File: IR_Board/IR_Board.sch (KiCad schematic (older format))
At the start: 16 parts, among them J1 Conn_02x08_Row_Letter_First, U1 TSSP58038, U10 TSSP58038, U11 TSSP58038, U12 TSSP58038, U13 TSSP58038, U14 TSSP58038, U2 TSSP58038, U3 TSSP58038, U4 TSSP58038, U5 TSSP58038, U6 TSSP58038, U7 TSSP58038, U8 TSSP58038, U9 TSSP58038

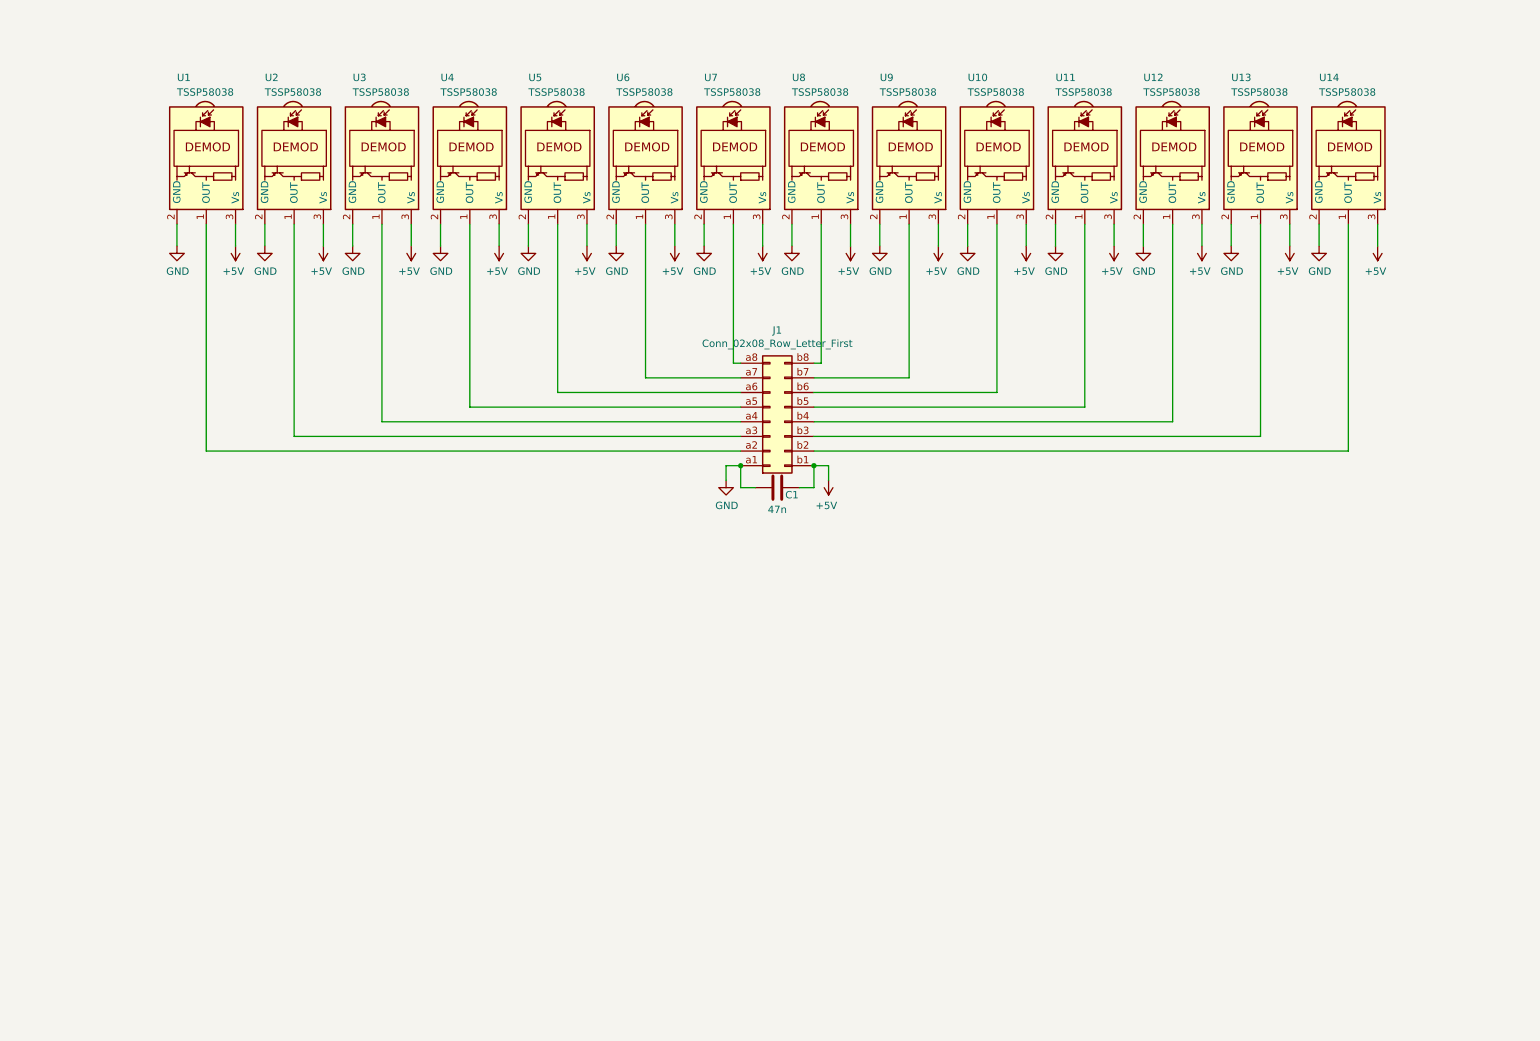
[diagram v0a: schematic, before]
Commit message: Started Light PCB
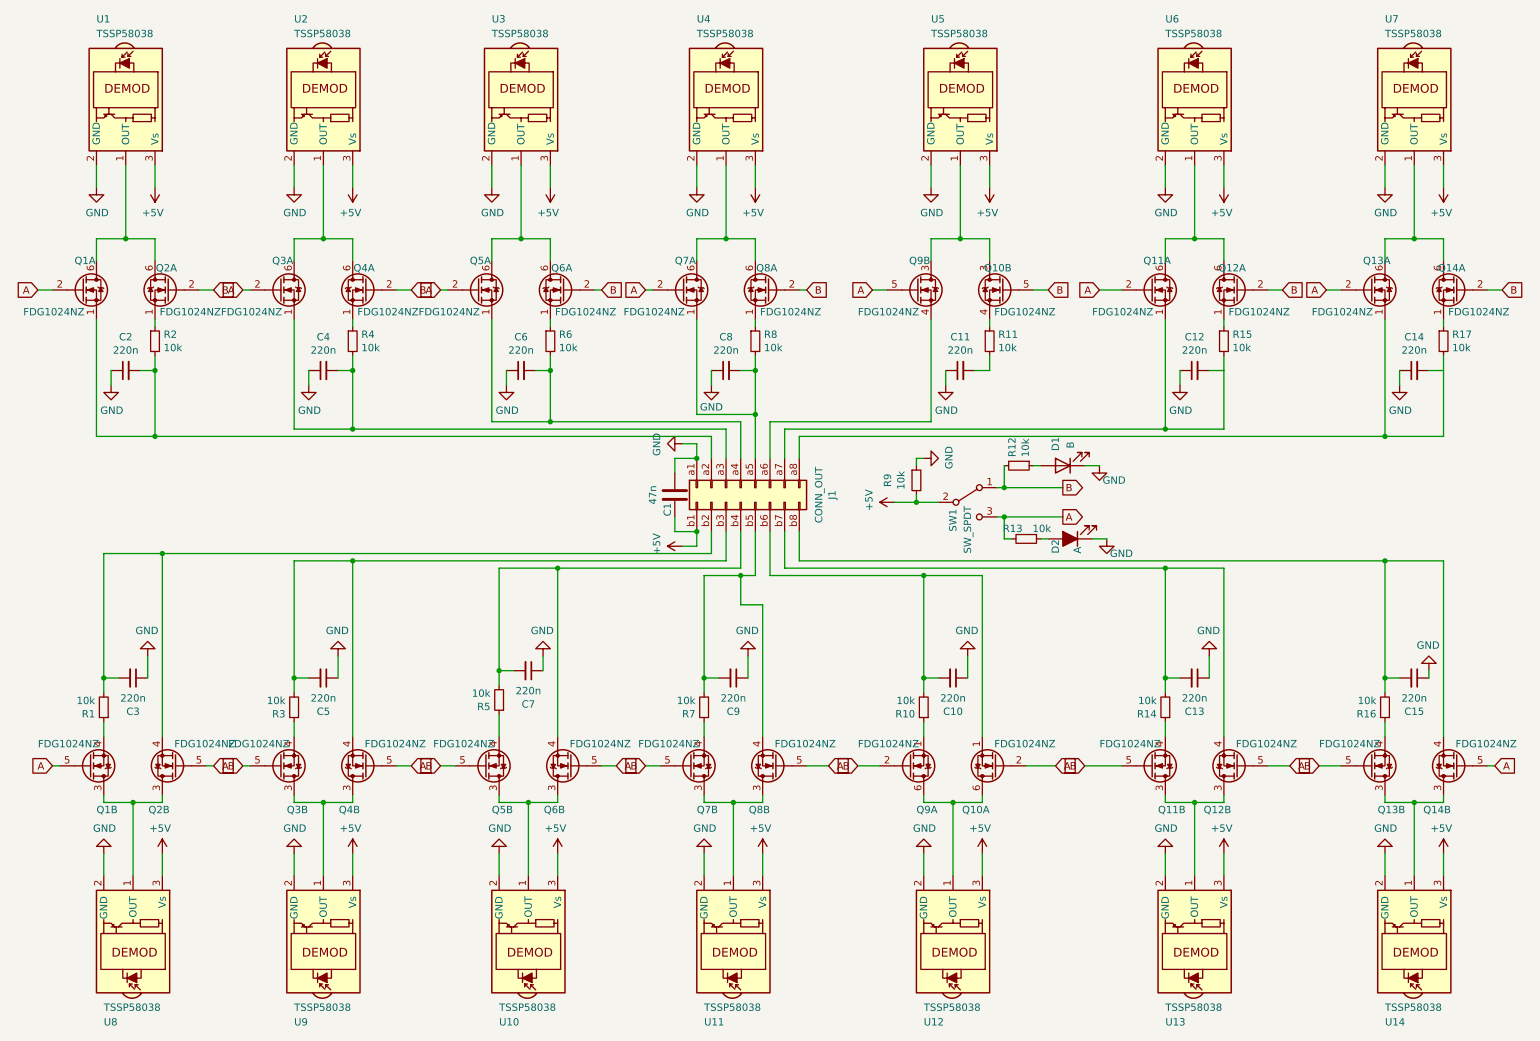
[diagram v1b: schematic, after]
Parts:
- added C10, C11, C12, C13, C14, C15, C2, C3, C4, C5, C6, C7, C8, C9: 220n, Capacitor_SMD:C_0603_1608Metric_Pad1.08x0.95mm_HandSolder, symbol Device:C_Small
- added D1: B, LED_SMD:LED_0805_2012Metric_Pad1.15x1.40mm_HandSolder, symbol Device:LED
- added D2: A, LED_SMD:LED_0805_2012Metric_Pad1.15x1.40mm_HandSolder, symbol Device:LED_ALT
- added Q1, Q10, Q11, Q12, Q13, Q14, Q2, Q3, Q4, Q5, Q6, Q7, Q8, Q9: FDG1024NZ, Package_TO_SOT_SMD:SOT-363_SC-70-6, symbol Transistor_FET:FDG1024NZ
- added R1, R10, R11, R12, R13, R14, R15, R16, R17, R2, R3, R4, R5, R6, R7, R8, R9: 10k, Resistor_SMD:R_0603_1608Metric_Pad0.98x0.95mm_HandSolder, symbol Device:R_Small
- added SW1: SW_SPDT, Connector_PinHeader_2.54mm:PinHeader_1x03_P2.54mm_Vertical, symbol Switch:SW_SPDT
- C1: footprint Capacitor_SMD:C_0603_1608Metric_Pad1.05x0.95mm_HandSolder -> Capacitor_SMD:C_0603_1608Metric_Pad1.08x0.95mm_HandSolder
- J1: value Conn_02x08_Row_Letter_First -> CONN_OUT
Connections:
- net +5V: now also R9.2, SW1.2 (B)
- net GND: now also C10.1, C11.1, C12.1, C13.1, C14.1, C15.1, C2.1, C3.1, C4.1, C5.1, C6.1, C7.1, C8.1, C9.1, D1.1 (K), D2.1 (K), R9.1
- net at U1.1 (OUT): now also Q1.6 (D), Q2.6 (D); no longer J1.a2 (Pin_a2)
- net at U2.1 (OUT): now also Q3.6 (D), Q4.6 (D); no longer J1.a3 (Pin_a3)
- net at U3.1 (OUT): now also Q5.6 (D), Q6.6 (D); no longer J1.a4 (Pin_a4)
- net at U4.1 (OUT): now also Q7.6 (D), Q8.6 (D); no longer J1.a5 (Pin_a5)
- net at U5.1 (OUT): now also Q10.3 (D), Q9.3 (D); no longer J1.a6 (Pin_a6)
- net at U6.1 (OUT): now also Q11.6 (D), Q12.6 (D); no longer J1.a7 (Pin_a7)
- net at U7.1 (OUT): now also Q13.6 (D), Q14.6 (D); no longer J1.a8 (Pin_a8)
- net at U8.1 (OUT): now also Q1.3 (D), Q2.3 (D); no longer J1.b8 (Pin_b8)
- net at U9.1 (OUT): now also Q3.3 (D), Q4.3 (D); no longer J1.b7 (Pin_b7)
- net at U10.1 (OUT): now also Q5.3 (D), Q6.3 (D); no longer J1.b6 (Pin_b6)
- net at U11.1 (OUT): now also Q7.3 (D), Q8.3 (D); no longer J1.b5 (Pin_b5)
- net at U12.1 (OUT): now also Q10.6 (D), Q9.6 (D); no longer J1.b4 (Pin_b4)
- net at U13.1 (OUT): now also Q11.3 (D), Q12.3 (D); no longer J1.b3 (Pin_b3)
- net at U14.1 (OUT): now also Q13.3 (D), Q14.3 (D); no longer J1.b2 (Pin_b2)
- new net: C2.2, J1.a2 (Pin_a2), Q1.1 (S), R2.2
- new net: C4.2, J1.a3 (Pin_a3), Q3.1 (S), R4.2
- new net: C6.2, J1.a4 (Pin_a4), Q5.1 (S), R6.2
- new net: C8.2, J1.a5 (Pin_a5), Q7.1 (S), R8.2
- new net: J1.a6 (Pin_a6), Q9.4 (S)
- new net: J1.a7 (Pin_a7), Q11.1 (S), R15.2
- new net: J1.a8 (Pin_a8), Q13.1 (S), R17.2
- new net: C3.2, J1.b2 (Pin_b2), Q2.4 (S), R1.2
- new net: C5.2, J1.b3 (Pin_b3), Q4.4 (S), R3.2
- new net: C7.2, J1.b4 (Pin_b4), Q6.4 (S), R5.2
- new net: C9.2, J1.b5 (Pin_b5), Q8.4 (S), R7.2
- new net: C10.2, J1.b6 (Pin_b6), Q10.1 (S), R10.2
- new net: C13.2, J1.b7 (Pin_b7), Q12.4 (S), R14.2
- new net: C15.2, J1.b8 (Pin_b8), Q14.4 (S), R16.2
- new net: Q2.1 (S), R2.1
- new net: Q4.1 (S), R4.1
- new net: Q6.1 (S), R6.1
- new net: Q8.1 (S), R8.1
- new net: Q10.4 (S), R11.1
- new net: Q12.1 (S), R15.1
- new net: Q14.1 (S), R17.1
- new net: Q13.4 (S), R16.1
- new net: Q11.4 (S), R14.1
- new net: Q9.1 (S), R10.1
- new net: Q7.4 (S), R7.1
- new net: Q5.4 (S), R5.1
- new net: Q3.4 (S), R3.1
- new net: Q1.4 (S), R1.1
- new net: C11.2, R11.2
- new net: D2.2 (A), R13.1
- new net: D1.2 (A), R12.1
- new net A: Q1.2 (G), Q1.5 (G), Q10.2 (G), Q11.2 (G), Q12.5 (G), Q13.2 (G), Q14.5 (G), Q2.5 (G), Q3.2 (G), Q4.5 (G), Q5.2 (G), Q6.5 (G), Q7.2 (G), Q8.5 (G), Q9.5 (G), R13.2, SW1.3 (C)
- new net B: Q10.5 (G), Q11.5 (G), Q12.2 (G), Q13.5 (G), Q14.2 (G), Q2.2 (G), Q3.5 (G), Q4.2 (G), Q5.5 (G), Q6.2 (G), Q7.5 (G), Q8.2 (G), Q9.2 (G), R12.2, SW1.1 (A)
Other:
- moved on the sheet: C1, J1, U1, U10, U11, U12, U13, U14, U2, U3, U4, U5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
